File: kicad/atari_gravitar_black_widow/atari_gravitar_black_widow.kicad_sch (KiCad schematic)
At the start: 0 parts

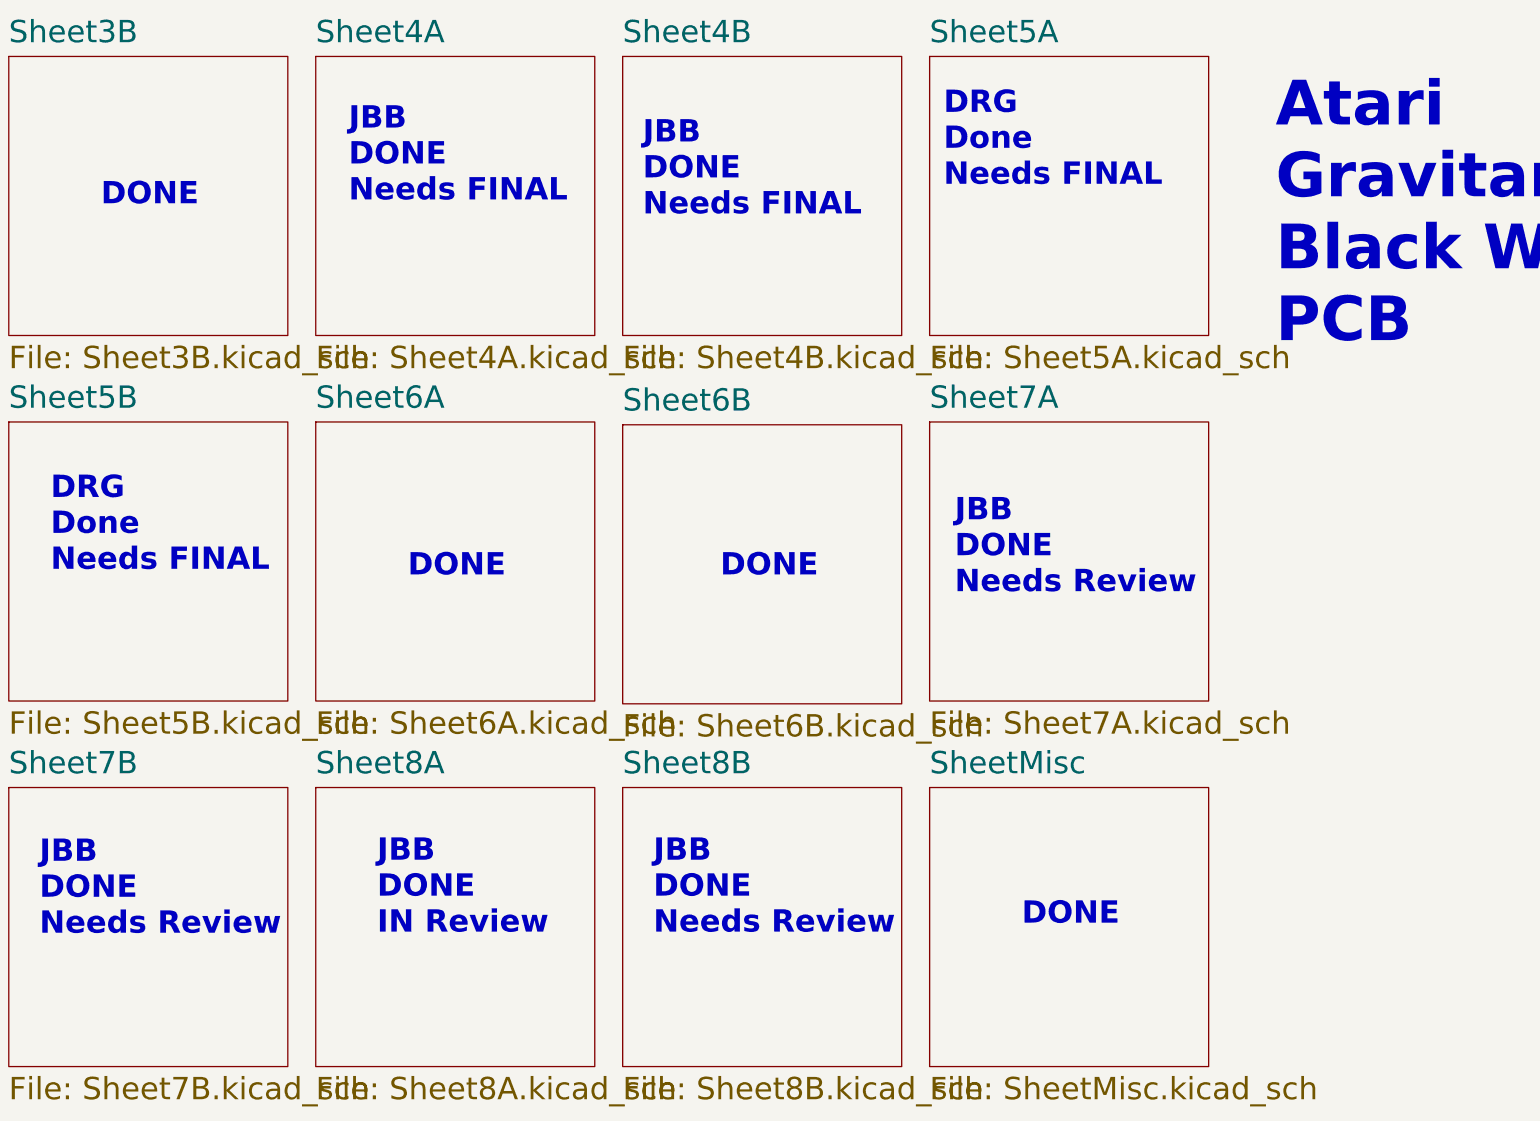
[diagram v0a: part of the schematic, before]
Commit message: reviewed first two sheets
see notes on individual sheets
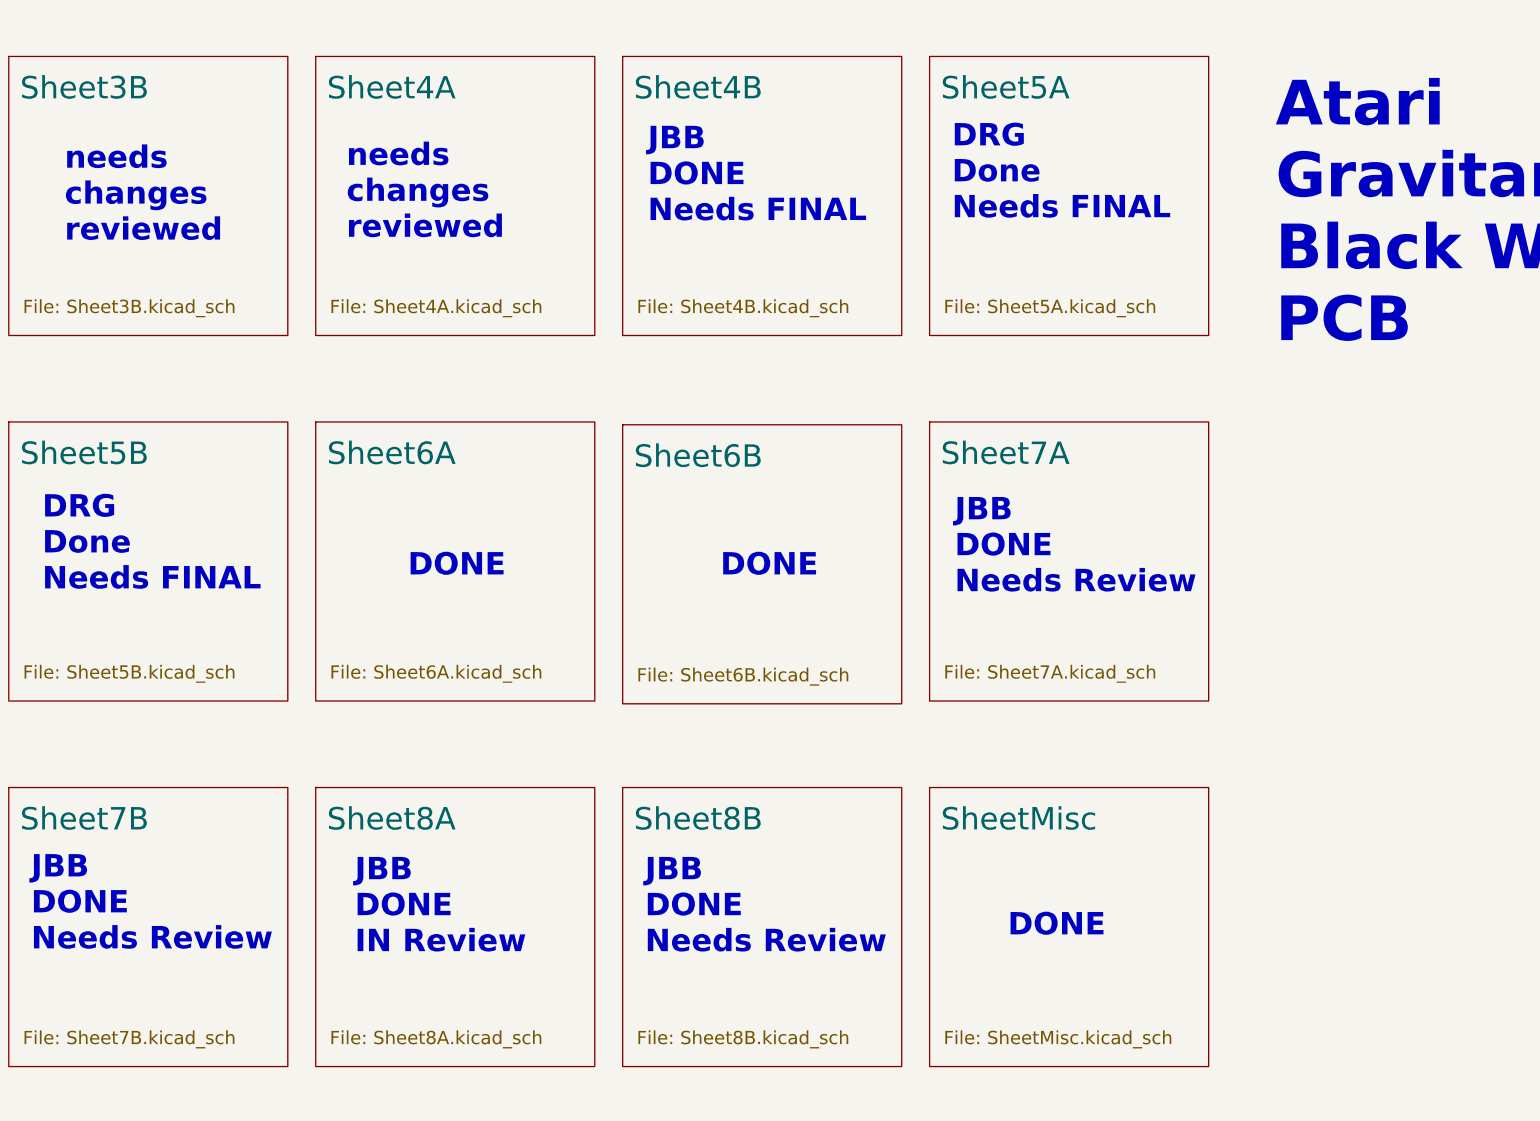
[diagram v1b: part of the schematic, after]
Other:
- note added: "needs changes reviewed"
